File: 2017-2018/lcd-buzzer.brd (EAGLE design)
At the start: 160 x 100 mm, 15 parts, among them U1 ATMEGA328P-MUR, U2 DRV2605YZFR, U3 74HC595PW, U4 74HC595PW, U5 74HC595PW, U6 74HC595PW

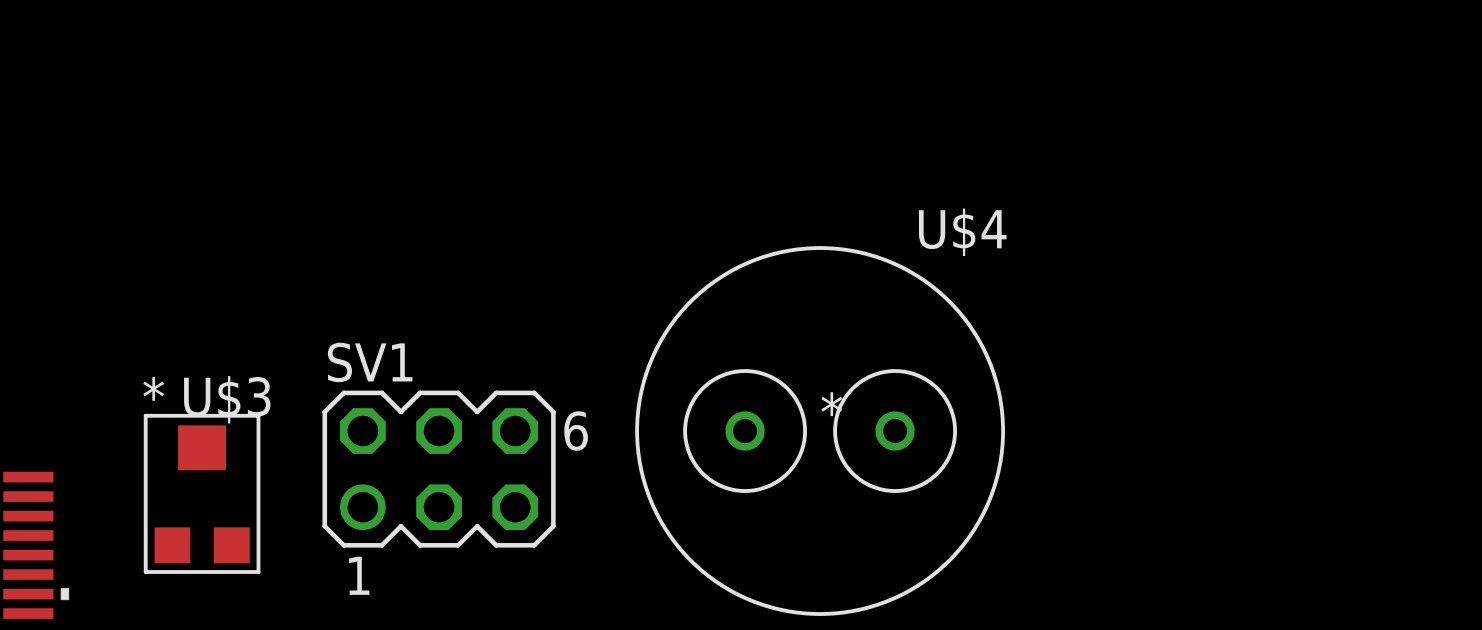
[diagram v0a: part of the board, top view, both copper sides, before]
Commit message: Separate clocks for registers
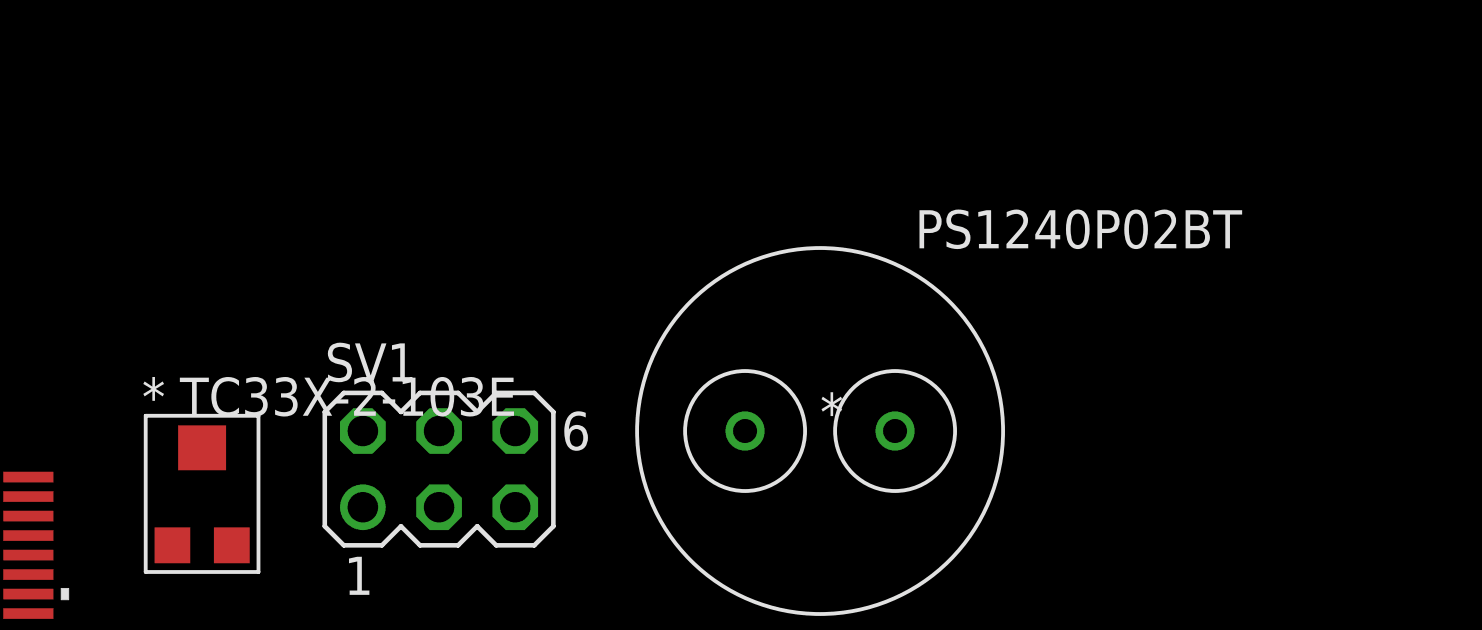
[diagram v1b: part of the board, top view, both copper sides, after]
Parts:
- renumbered U$3 to TC33X-2-103E, U$4 to PS1240P02BT
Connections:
- removed net SHIFT_CLK: U1.31, U3.12, U4.12, U5.12, U6.12
- removed net STORAGE_CLK: U1.30, U3.11, U4.11, U5.11, U6.11
- new net SHIFT_CLK1: U1.9, U3.12
- new net SHIFT_CLK2: U1.10, U4.12
- new net SHIFT_CLK3: U1.11, U5.12
- new net SHIFT_CLK4: U1.12, U6.12
- new net STORAGE_CLK1: U1.13, U3.11
- new net STORAGE_CLK2: U1.14, U4.11
- new net STORAGE_CLK3: U1.30, U5.11
- new net STORAGE_CLK4: U1.31, U6.11
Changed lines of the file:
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@@
 <element name="U$1" library="rgb-led" package="GS-14-2180" value="MICRO-USB" x="-53.34" y="57.15"/>
 <element name="U$2" library="lcd-buzzer" package="S401C39TR" value="LCD-S401C39TR" x="-63.5" y="1.27"/>
-<element name="U$3" library="lcd-buzzer" package="TC33X-2-103E" value="TC33X" x="-53.34" y="33.02"/>
-<element name="U$4" library="lcd-buzzer" package="PS1240P02BT" value="PS1240P02BT" x="-30.48" y="38.1"/>
+<element name="TC33X-2-103E" library="lcd-buzzer" package="TC33X-2-103E" value="TC33X" x="-53.34" y="33.02"/>
+<element name="PS1240P02BT" library="lcd-buzzer" package="PS1240P02BT" value="PS1240P02BT" x="-30.48" y="38.1"/>
 <element name="U1" library="lcd-buzzer" package="32M1-A" value="ATMEGA328P-MUR" x="-43.18" y="58.42">
 <attribute name="MANUFACTURER_PART_NUMBER" value="ATMEGA328PMUR" x="-43.18" y="58.42" size="1.778" layer="27" display="off"/>
@@
 <contactref element="U1" pad="4"/>
 <contactref element="U1" pad="18"/>
-<contactref element="U$3" pad="CCW"/>
+<contactref element="TC33X-2-103E" pad="CCW"/>
 <contactref element="SV1" pad="2"/>
 <wire x1="-15.24" y1="63" x2="-15.74" y2="64" width="0" layer="19" extent="1-1"/>
@@
 <contactref element="U1" pad="3"/>
 <contactref element="U1" pad="21"/>
-<contactref element="U$3" pad="CW"/>
+<contactref element="TC33X-2-103E" pad="CW"/>
 <contactref element="SV1" pad="6"/>
 <wire x1="-15.74" y1="63.5" x2="-14.74" y2="63.5" width="0" layer="19" extent="1-1"/>
@@
 <wire x1="-62.5094" y1="32.015" x2="-56.8706" y2="34.614996875" width="0" layer="19" extent="1-1"/>
 </signal>
-<signal name="SHIFT_CLK">
-<contactref element="U3" pad="12"/>
-<contactref element="U4" pad="12"/>
-<contactref element="U5" pad="12"/>
+<signal name="SHIFT_CLK4">
 <contactref element="U6" pad="12"/>
+<contactref element="U1" pad="12"/>
+<wire x1="-43.43" y1="56.0197" x2="-32.7406" y2="56.825" width="0" layer="19" extent="1-1"/>
+</signal>
+<signal name="STORAGE_CLK4">
+<contactref element="U6" pad="11"/>
 <contactref element="U1" pad="31"/>
-<wire x1="-23.8506" y1="56.825" x2="-14.9606" y2="56.825" width="0" layer="19" extent="1-1"/>
-<wire x1="-32.7406" y1="56.825" x2="-23.8506" y2="56.825" width="0" layer="19" extent="1-1"/>
-<wire x1="-44.43" y1="60.8203" x2="-32.7406" y2="56.825" width="0" layer="19" extent="1-1"/>
-<wire x1="-56.8706" y1="33.965" x2="-44.43" y2="60.8203" width="0" layer="19" extent="1-1"/>
-</signal>
-<signal name="STORAGE_CLK">
-<contactref element="U3" pad="11"/>
-<contactref element="U4" pad="11"/>
-<contactref element="U5" pad="11"/>
-<contactref element="U6" pad="11"/>
-<contactref element="U1" pad="30"/>
-<wire x1="-23.8506" y1="56.175" x2="-14.9606" y2="56.175" width="0" layer="19" extent="1-1"/>
-<wire x1="-32.7406" y1="56.175" x2="-23.8506" y2="56.175" width="0" layer="19" extent="1-1"/>
-<wire x1="-43.93" y1="60.8203" x2="-32.7406" y2="56.175" width="0" layer="19" extent="1-1"/>
-<wire x1="-56.8706" y1="33.315" x2="-43.93" y2="60.8203" width="0" layer="19" extent="1-1"/>
+<wire x1="-44.43" y1="60.8203" x2="-32.7406" y2="56.175" width="0" layer="19" extent="1-1"/>
 </signal>
 <signal name="SFT1">
@@
 <signal name="LRA/ERM+">
 <contactref element="U2" pad="A3"/>
-<contactref element="U$4" pad="P$1"/>
+<contactref element="PS1240P02BT" pad="P$1"/>
 <wire x1="-32.98" y1="38.1" x2="-14.74" y2="64" width="0" layer="19" extent="1-1"/>
 </signal>
 <signal name="LRA/ERM-">
 <contactref element="U2" pad="C3"/>
-<contactref element="U$4" pad="P$2"/>
+<contactref element="PS1240P02BT" pad="P$2"/>
 <wire x1="-27.98" y1="38.1" x2="-14.74" y2="63" width="0" layer="19" extent="1-1"/>
 </signal>
@@
 </signal>
 <signal name="DIVIDED">
-<contactref element="U$3" pad="WIPER"/>
+<contactref element="TC33X-2-103E" pad="WIPER"/>
 <contactref element="U$2" pad="P$1"/>
 <contactref element="U$2" pad="P$40"/>
@@
 <wire x1="-51.0794" y1="37.5412" x2="-63.5" y2="25.908" width="0" layer="19" extent="1-1"/>
 </signal>
+<signal name="SHIFT_CLK1">
+<contactref element="U3" pad="12"/>
+<contactref element="U1" pad="9"/>
+<wire x1="-44.93" y1="56.0197" x2="-56.8706" y2="33.965" width="0" layer="19" extent="1-1"/>
+</signal>
+<signal name="STORAGE_CLK1">
+<contactref element="U3" pad="11"/>
+<contactref element="U1" pad="13"/>
+<wire x1="-42.93" y1="56.0197" x2="-56.8706" y2="33.315" width="0" layer="19" extent="1-1"/>
+</signal>
+<signal name="STORAGE_CLK2">
+<contactref element="U4" pad="11"/>
+<contactref element="U1" pad="14"/>
+<wire x1="-42.43" y1="56.0197" x2="-14.9606" y2="56.175" width="0" layer="19" extent="1-1"/>
+</signal>
+<signal name="SHIFT_CLK2">
+<contactref element="U4" pad="12"/>
+<contactref element="U1" pad="10"/>
+<wire x1="-44.43" y1="56.0197" x2="-14.9606" y2="56.825" width="0" layer="19" extent="1-1"/>
+</signal>
+<signal name="STORAGE_CLK3">
+<contactref element="U5" pad="11"/>
+<contactref element="U1" pad="30"/>
+<wire x1="-43.93" y1="60.8203" x2="-23.8506" y2="56.175" width="0" layer="19" extent="1-1"/>
+</signal>
+<signal name="SHIFT_CLK3">
+<contactref element="U5" pad="12"/>
+<contactref element="U1" pad="11"/>
+<wire x1="-43.93" y1="56.0197" x2="-23.8506" y2="56.825" width="0" layer="19" extent="1-1"/>
+</signal>
 </signals>
